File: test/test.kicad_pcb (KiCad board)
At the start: 2 copper layers, 20.3 x 20.3 mm, 5 parts

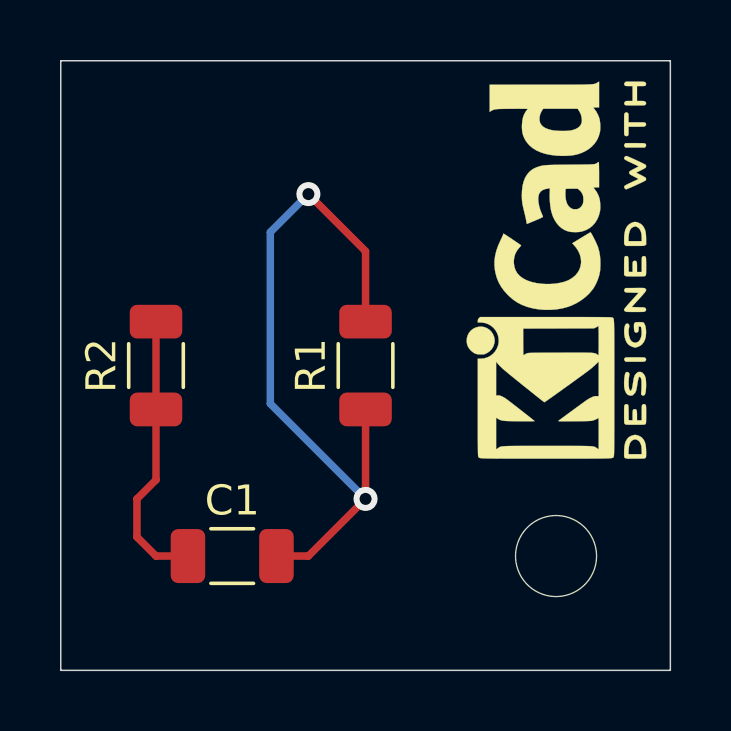
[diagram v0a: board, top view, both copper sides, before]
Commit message: changed test project
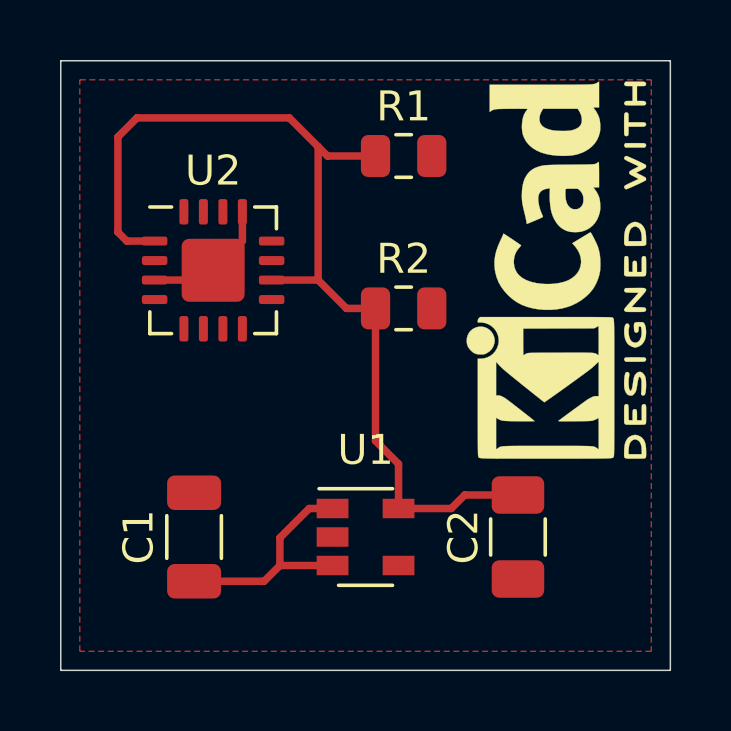
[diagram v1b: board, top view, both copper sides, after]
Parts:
- removed H1: MountingHole, MountingHole:MountingHole_2.7mm
- added C2: 100nF, Capacitor_SMD:C_1206_3216Metric, F.Cu at (134.6, 104.8)
- added U1: TLV70233_SOT23-5, Package_TO_SOT_SMD:SOT-23-5, F.Cu at (129.5, 104.8)
- added U2: FT230XQ, Package_DFN_QFN:QFN-16-1EP_4x4mm_P0.65mm_EP2.1x2.1mm, F.Cu at (124.5, 95.9)
- R1, R2: value 100 -> R; footprint Resistor_SMD:R_1206_3216Metric -> Resistor_SMD:R_0805_2012Metric
- moved R2 8.47 mm to (130.8, 97.2), turned to 0 degrees
- moved R1 7.10 mm to (130.8, 92.1), turned to 0 degrees
- moved C1 1.42 mm to (123.8, 104.8), turned to 90 degrees
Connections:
- C1 pad 2: Net-(C1-Pad2) -> GND
- R1 pad 1: Net-(C1-Pad2) -> +3V3
- R1 pad 2: Net-(C1-Pad2) -> GND
- R2 pad 1: Net-(C1-Pad1) -> +3V3
- R2 pad 2: Net-(C1-Pad1) -> GND
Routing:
- net +3V3: track 0.00 -> 33.4 mm
- net Net-(C1-Pad2): track 24.0 -> 0.00 mm, vias 2 -> 0
- net GND: track 0.00 -> 4.44 mm
- net Net-(C1-Pad1): track 10.1 -> 7.92 mm
- added copper zone on F.Cu, net GND
